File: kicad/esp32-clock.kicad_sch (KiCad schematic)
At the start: 11 parts, among them SW1 RESET, SW2 BOOT, U1 ESP-12E

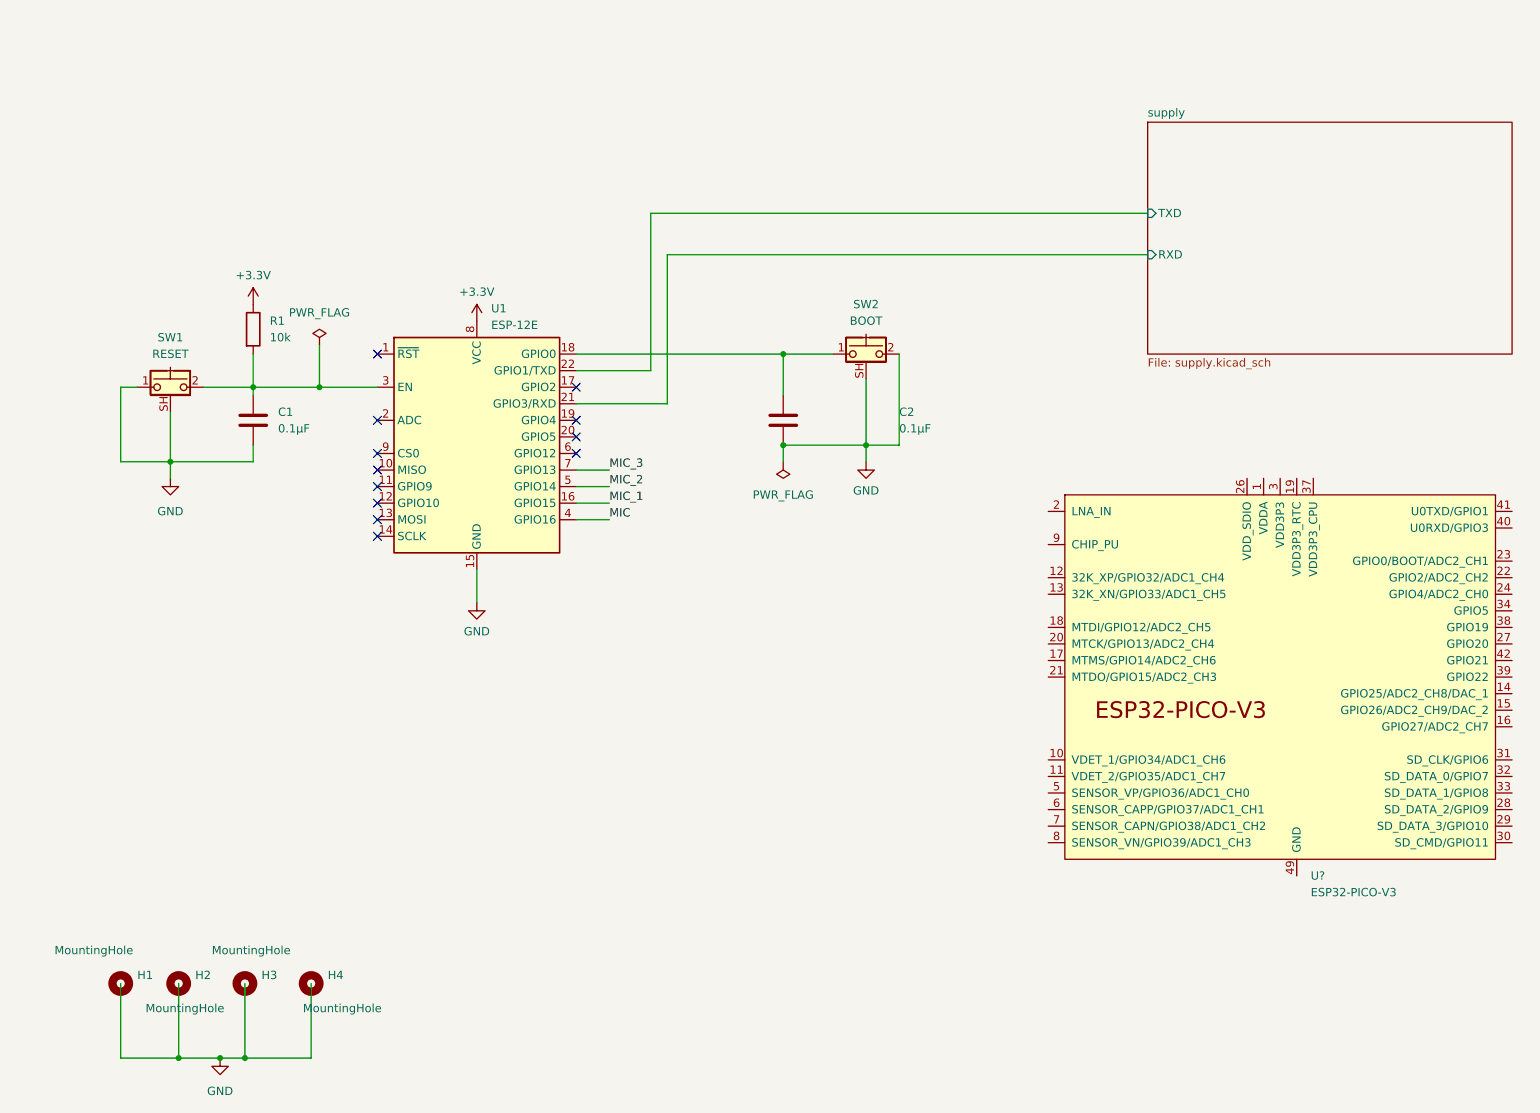
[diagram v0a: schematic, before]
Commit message: init
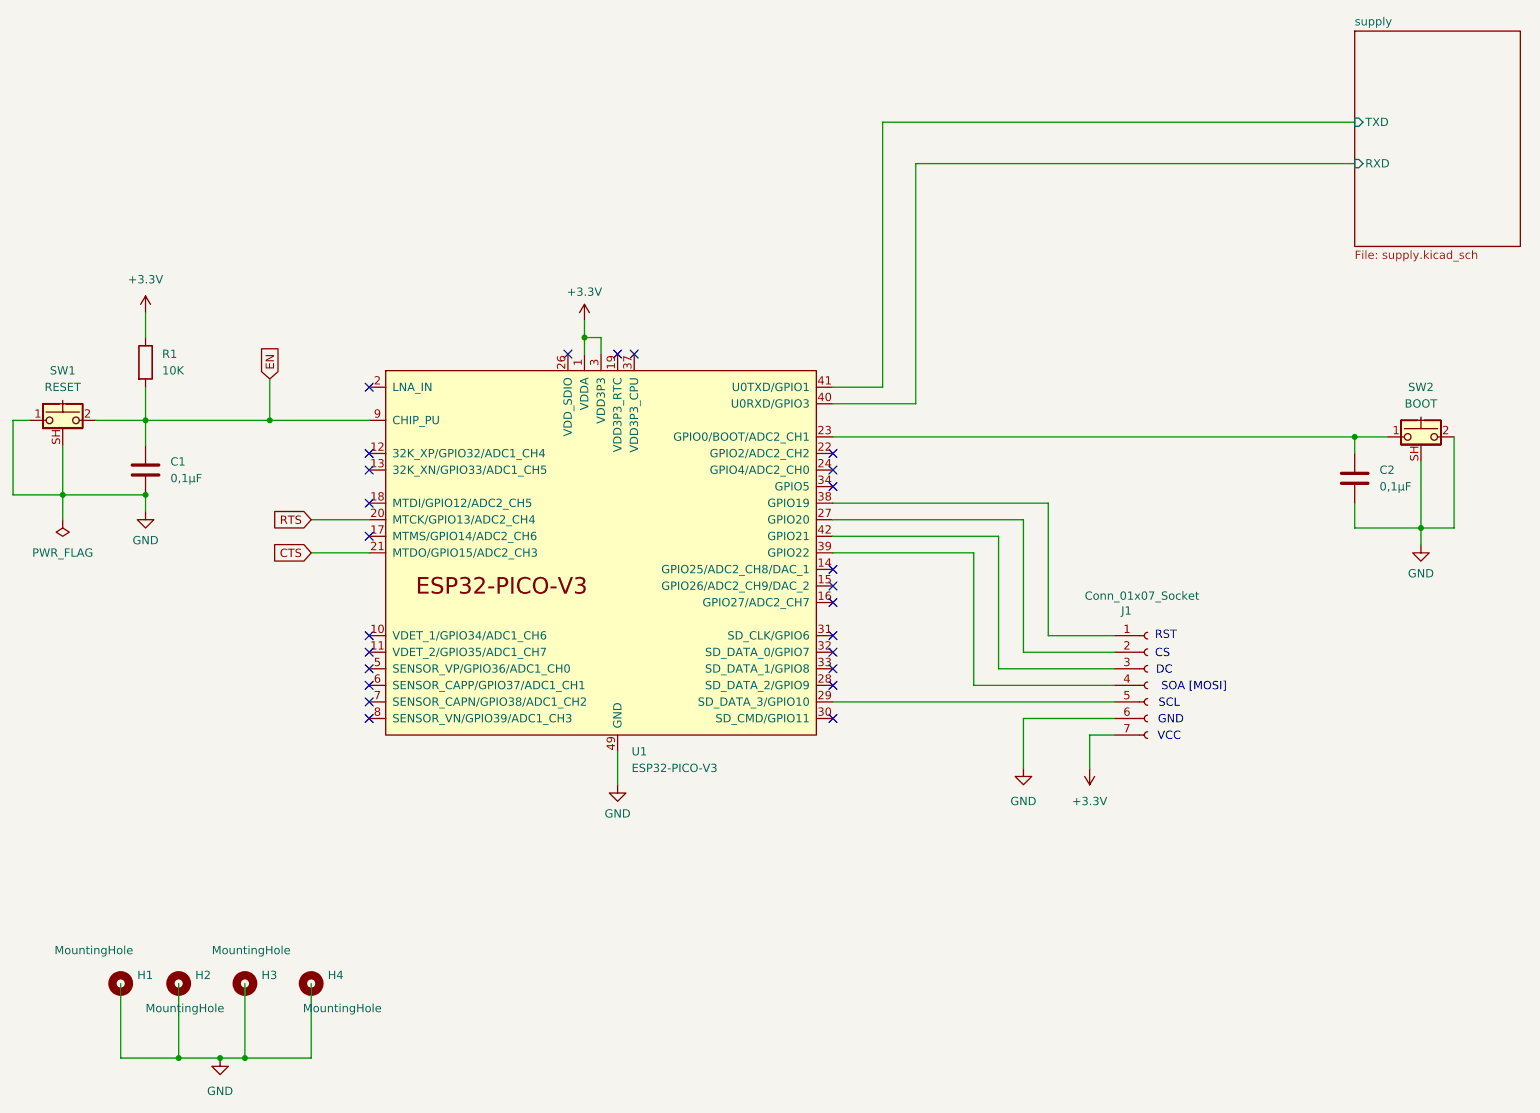
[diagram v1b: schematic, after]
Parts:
- removed U1: ESP-12E, RF_Module:ESP-12E, symbol RF_Module:ESP-12E
- added J1: Conn_01x07_Socket, Connector_PinSocket_2.54mm:PinSocket_1x07_P2.54mm_Vertical, symbol Connector:Conn_01x07_Socket
- C1, C2: value 0.1µF -> 0,1µF
- R1: value 10k -> 10K; LCSC C1489 -> (none)
- gave numbers to parts that had none: 1
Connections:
- net +3.3V: now also U1.1 (VDDA), U1.3 (VDD3P3), U1.4 (VDD3P3), U1.43 (VDDA), U1.46 (VDDA), J1.7 (Pin_7)
- net GND: now also U1.49 (GND), J1.6 (Pin_6)
- net supply/RXD: now also U1.40 (U0RXD/GPIO3)
- net supply/TXD: now also U1.41 (U0TXD/GPIO1)
- net at C2.1, SW2.1: now also U1.23 (GPIO0/BOOT/ADC2_CH1)
- net EN: now reaches C1.1, R1.2, SW1.2
- net EN: now also U1.9 (CHIP_PU)
- net RTS: now reaches U1.20 (MTCK/GPIO13/ADC2_CH4)
- net CTS: now reaches U1.21 (MTDO/GPIO15/ADC2_CH3)
- net at U1.27 (GPIO20): now also J1.2 (Pin_2)
- net at U1.29 (SD_DATA_3/GPIO10): now also J1.5 (Pin_5)
- net at U1.38 (GPIO19): now also J1.1 (Pin_1)
- net at U1.39 (GPIO22): now also J1.4 (Pin_4)
- net at U1.42 (GPIO21): now also J1.3 (Pin_3)
- no-connect marks 12 -> 25
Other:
- note added: "CS"
- note added: "DC"
- note added: "GND"
- note added: "RST"
- note added: "SCL"
- note added: "SOA [MOSI]"
- note added: "VCC"
- moved on the sheet: SW1, SW2, U1
